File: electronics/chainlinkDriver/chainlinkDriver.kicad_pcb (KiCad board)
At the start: 2 copper layers, 198.1 x 30.5 mm, 56 parts, among them J10 Sensor, J11 Sensor, J12 Motor, J14 Sensor, J16 Power, J18 Power, J19 IDC, J3 Motor, J5 Motor, J6 Motor, J7 Motor, J8 Sensor, J9 Sensor, U1 74HC595, U10 TPL7407L, U2 TPL7407L, U4 74HC165, U5 74HC595, U6 TPL7407L, U7 74HC595, U8 TPL7407L, U9 74HC595

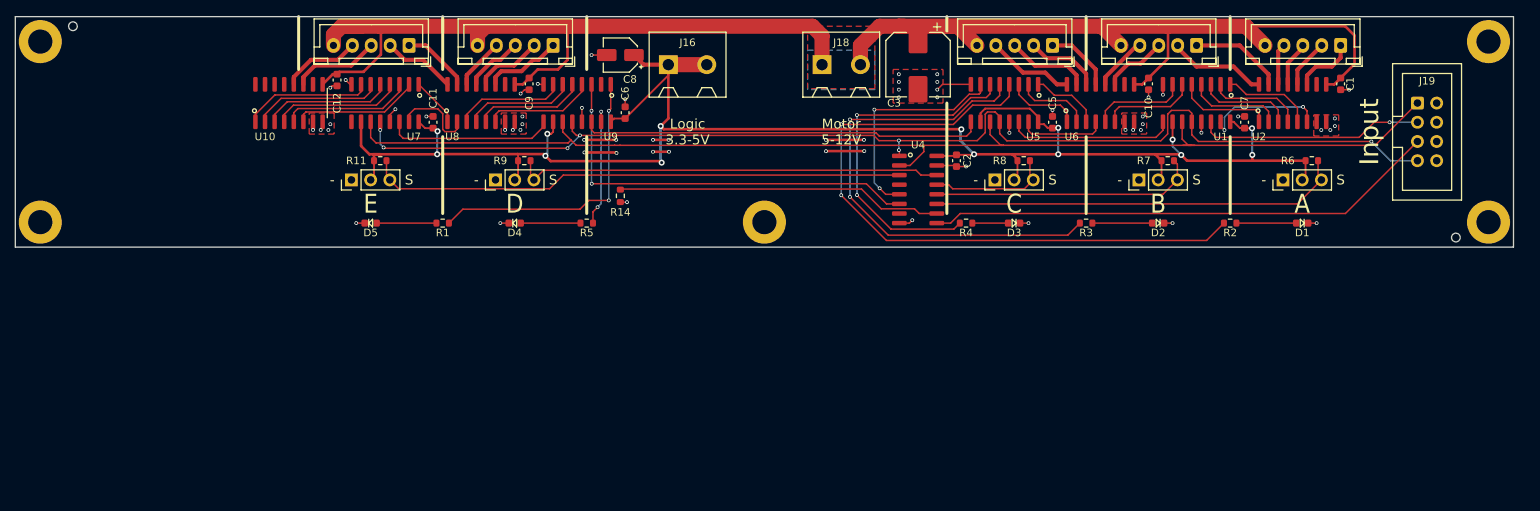
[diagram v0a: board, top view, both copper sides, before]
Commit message: design update
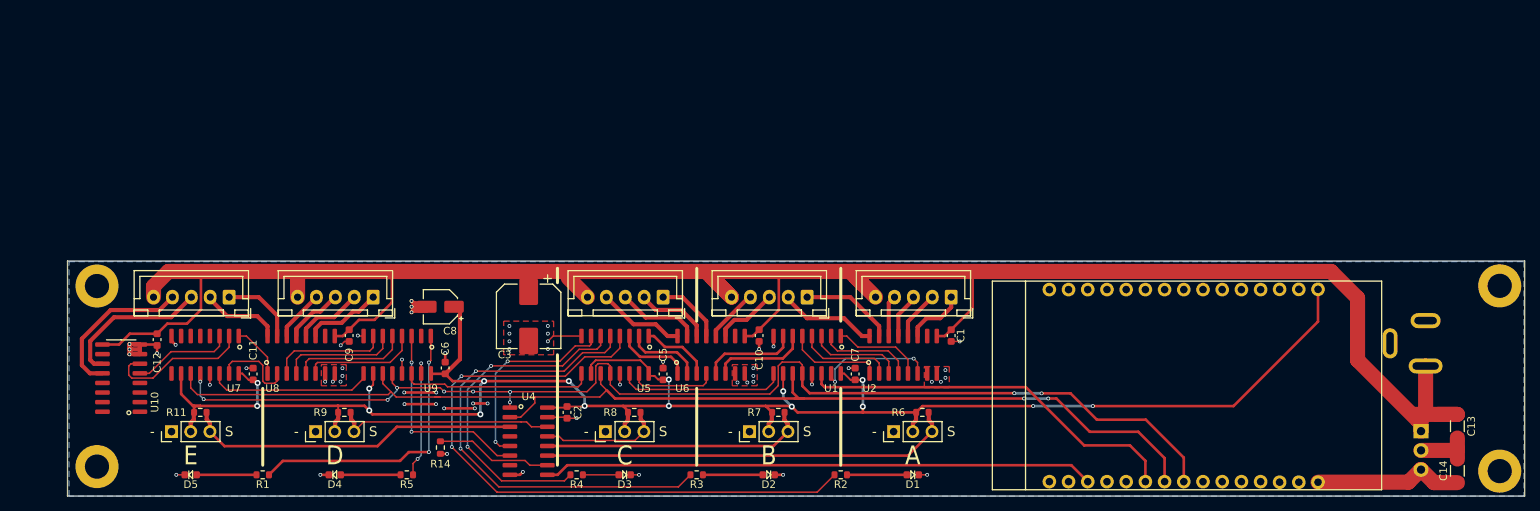
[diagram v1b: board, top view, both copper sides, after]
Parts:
- removed H5: MountingHole, MountingHole:MountingHole_3.2mm_M3_ISO7380_Pad
- removed H6, H7: MountingHole, JLCPCB:AssemblyToolingHole
- removed J16, J18: Power, ScrewTerminals:Generic-5.08-2P
- removed J19: IDC, ModifiedSymbols:IDC-Header_2x04_P2.54mm_Vertical
- added C13: 10uF, Capacitor_SMD:C_1206_3216Metric_Pad1.33x1.80mm_HandSolder, F.Cu at (216.1, 79.6)
- added C14: 22uF, Capacitor_SMD:C_1206_3216Metric_Pad1.33x1.80mm_HandSolder, F.Cu at (216.1, 85.5)
- added J1: Barrel_Jack_Switch, Library:PJ202, F.Cu at (217.4, 74.3)
- added U11: MyESP32, Library:MyESP32, F.Cu at (208.0, 91.0)
- added U3: LM7805_TO220, Library:TO-220-3_Vertical, F.Cu at (207.2, 75.0)
- moved J5 61.3 mm to (130.1, 62.5)
- moved U1 61.3 mm to (130.1, 70.1)
- moved C1 61.3 mm to (149.2, 67.6)
- moved C2 61.3 mm to (98.4, 77.7)
- moved C5 61.3 mm to (111.1, 72.7)
- moved C7 61.3 mm to (136.5, 72.7)
- moved J10 61.3 mm to (103.4, 80.3)
- moved J8 61.3 mm to (141.5, 80.3)
- moved J9 61.3 mm to (122.5, 80.3)
- moved R7 61.3 mm to (126.3, 77.7)
- moved U4 61.3 mm to (93.3, 81.5)
- moved U5 61.3 mm to (104.7, 70.1)
- moved C3 61.3 mm to (93.3, 65.0)
- moved D1 61.3 mm to (144.1, 86.0)
- moved D2 61.3 mm to (125.0, 86.0)
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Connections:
- net /CLOCK_IN renamed /CLOCK
- net /LATCH_IN renamed /LATCH
- U1 pad 14: /MOTOR_IN -> /MOTOR_DATA
- U4 pad 9: /SENSOR_OUT -> /SENSOR_DATA
- U7 pad 4: /MOTOR_F_PHASE_A -> unconnected-(U7-QE-Pad4)
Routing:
- net +12V: track 202.7 -> 277.4 mm
- net /SENSOR_DATA: track 0.00 -> 72.9 mm
- net /SENSOR_OUT: track 68.0 -> 0.00 mm
- net (no net): track 51.5 -> 0.00 mm
- net /MOTOR_DATA: track 0.00 -> 51.2 mm
- net /MOTOR_IN: track 29.8 -> 0.00 mm, vias 1 -> 0
- net /LOOPBACK_B: track 54.9 -> 27.0 mm
- net Net-(U5-QH'): track 53.2 -> 25.3 mm
- net /SENSOR_IN: track 43.2 -> 15.6 mm
- net /SENSOR_D: track 56.8 -> 29.7 mm
- net /SENSOR_E: track 71.3 -> 44.9 mm
- net +3.3V: track 231.6 -> 255.4 mm, vias 14 -> 16
- net +5V: track 0.00 -> 19.9 mm
- net /MOTOR_F_PHASE_A: track 17.2 -> 0.00 mm
- net GND: track 59.9 -> 73.0 mm, vias 62 -> 59
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- added copper zone on B.Cu, net GND
- removed copper zone on B.Cu, net +12V
- removed copper zone on F.Cu, net +12V
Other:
- board size 198.1 x 30.5 mm -> 192.7 x 31.1 mm
- board text removed: "Input"
- board text removed: "Logic 3.3-5V"
- board text removed: "Motor 5-12V"
